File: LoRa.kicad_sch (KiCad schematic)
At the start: 20 parts, among them U15 TPS7A4501DCQT, U16 ADM1176-1ARMZ-R7, U7 E22-900M30S

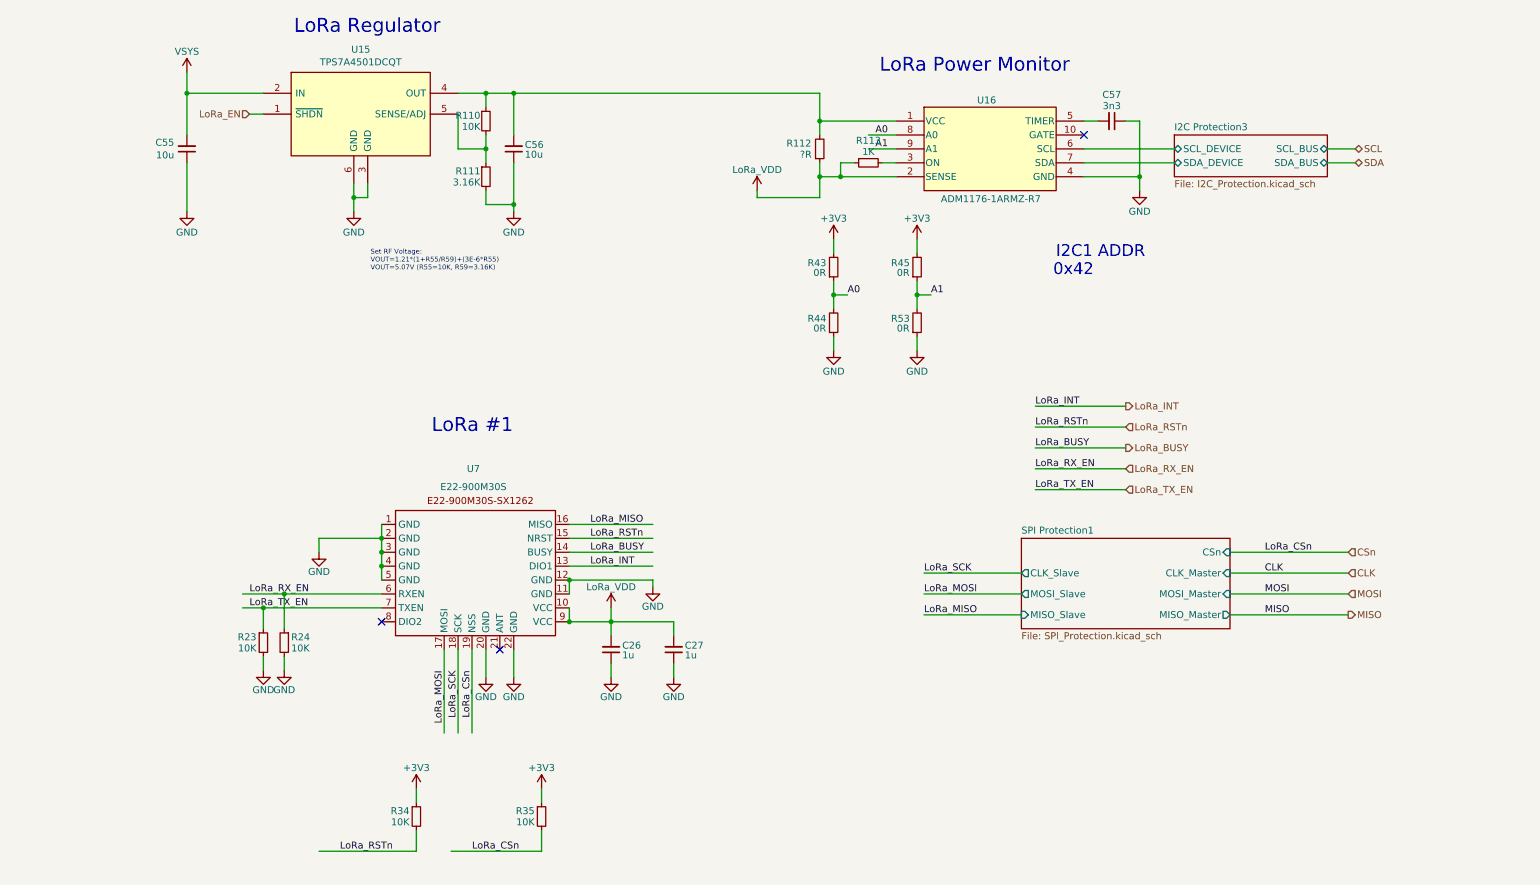
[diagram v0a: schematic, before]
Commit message: v3 partial schematic updates
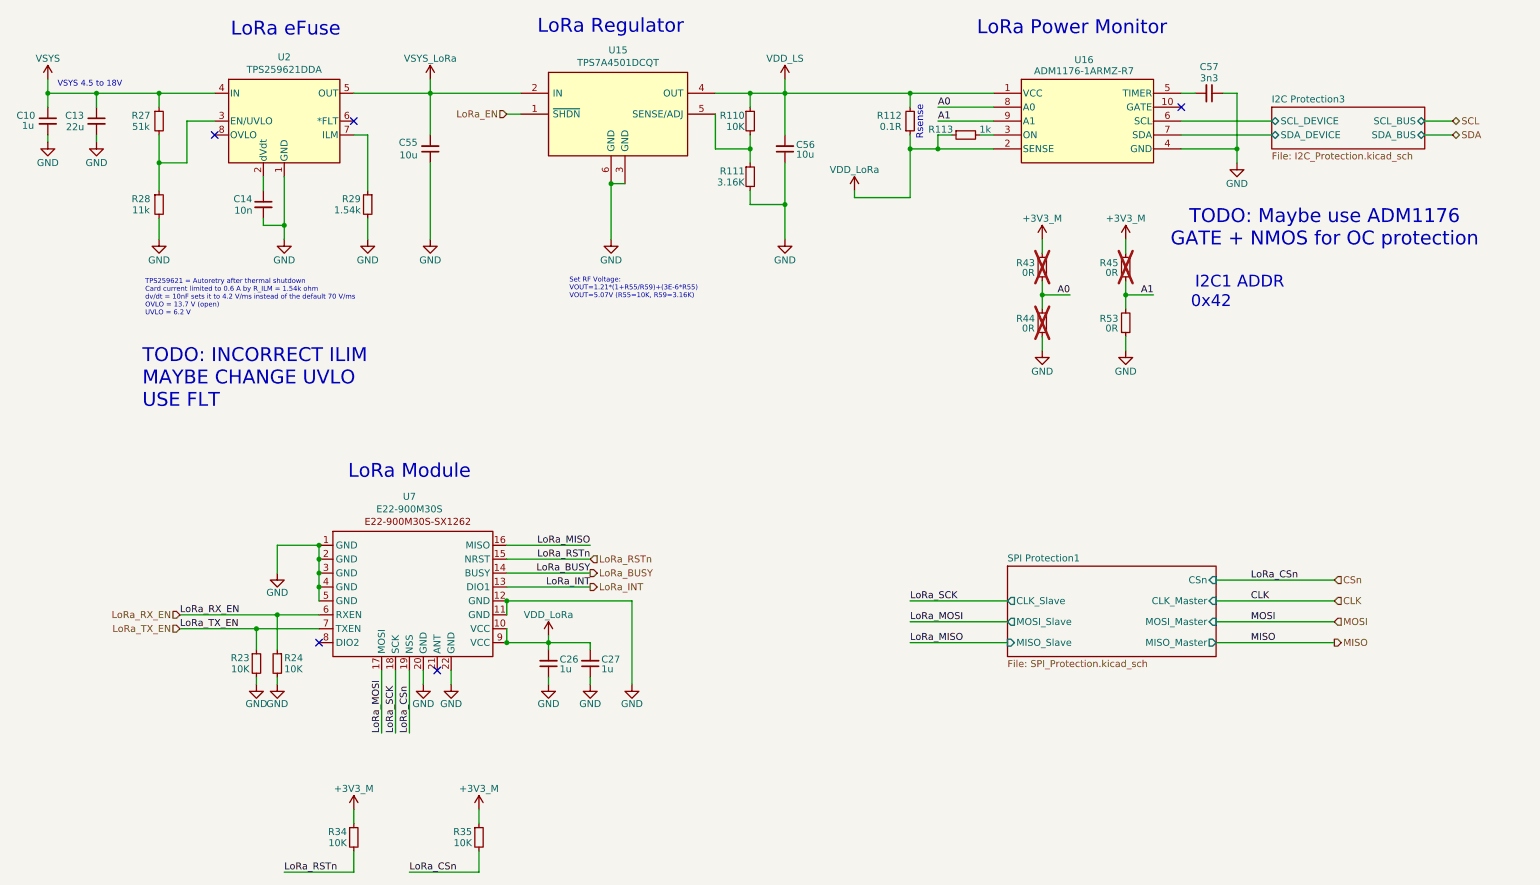
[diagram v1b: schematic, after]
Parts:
- added C10: 1u, Capacitor_SMD:C_0603_1608Metric, symbol Device:C_Small
- added C13: 22u, Capacitor_SMD:C_1210_3225Metric, symbol Device:C_Small
- added C14: 10n, Capacitor_SMD:C_0603_1608Metric, symbol Device:C_Small
- added R27: 51k, Resistor_SMD:R_0603_1608Metric, symbol Device:R_Small
- added R28: 11k, Resistor_SMD:R_0603_1608Metric, symbol Device:R_Small
- added R29: 1.54k, Resistor_SMD:R_0603_1608Metric, symbol Device:R_Small
- added U2: TPS259621DDA, Package_SO:Texas_R-PDSO-G8_EP2.95x4.9mm_Mask2.4x3.1mm_ThermalVias, symbol oresat-ics:TPS259621DDA
- R112: value ?R -> 0.1R
- R113: value 1K -> 1k
- R43, R44, R45: now not fitted
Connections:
- net GND: now also C10.2, C13.2, C14.2, R28.2, R29.2, U2.1 (GND), U2.9 (GND)
- net VSYS: now also C10.1, C13.1, R27.1, U2.4 (IN); no longer C55.2, U15.2 (IN)
- net VDD_LS: now reaches C56.2, R110.1, R112.2, U15.4 (OUT), U16.1 (VCC)
- net +3V3 renamed +3V3_M
- net LoRa_VDD renamed VDD_LoRa
- new net: C14.1, U2.2 (dVdt)
- new net: R27.2, R28.1, U2.3 (EN/UVLO)
- new net: R29.1, U2.7 (ILM)
- new net VSYS_LoRa: C55.2, U15.2 (IN), U2.5 (OUT)
- no-connect marks 3 -> 5
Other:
- note added: "LoRa Module"
- note added: "LoRa eFuse"
- note added: "Rsense"
- note added: "TODO: INCORRECT ILIM MAYBE CHANGE UVLO USE FLT"
- note added: "TODO: Maybe use ADM1176 GATE + NMOS for OC protection"
- note added: "TPS259621 = Autoretry after thermal shutdown Card current limited to 0.6 A by R_ILM = 1.54k ohm dv/dt = 10nF sets it to 4.2 V/ms instead of the default 70 V/ms OVLO = 13.7 V (open) UVLO = 6.2 V"
- note added: "VSYS 4.5 to 18V"
- note removed: "LoRa #1"
- moved on the sheet: C26, C27, C55, C56, C57, R110, R111, R112, R113, R23, R24, R34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
